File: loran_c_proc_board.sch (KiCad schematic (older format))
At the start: 28 parts, among them P101 Power, P102 Cortex SWD, P103 Clock board, U101 LD1117S33, U102 74AC14, U103 74AC14

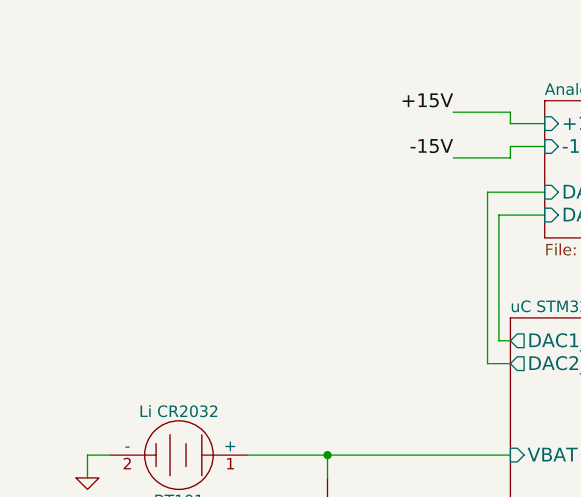
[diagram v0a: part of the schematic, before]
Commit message: Intermediate update #2: PCB routing/schematic tweaking in process
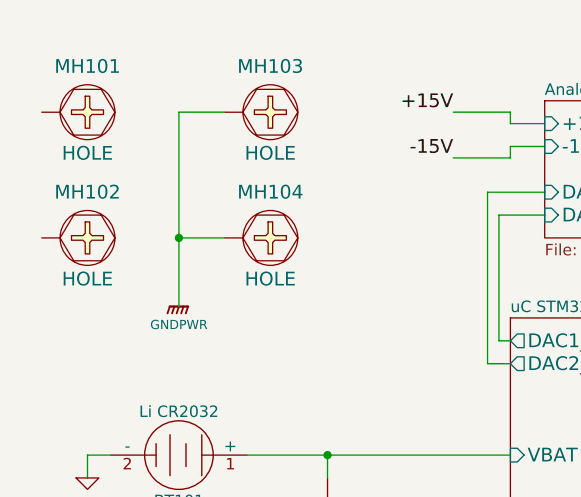
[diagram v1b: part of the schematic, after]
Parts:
- added MH101, MH102, MH103, MH104: HOLE, symbol HOLE
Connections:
- net GNDPWR: now also MH103.1, MH104.1
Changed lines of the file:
@@
 LIBS:transf
 LIBS:video
+LIBS:led_holder
 LIBS:loran_c_proc_board-cache
 EELAYER 24 0
@@
 	4900 1300 4900 1450
 Connection ~ 5300 1450
+$Comp
+L HOLE MH104
+U 1 1 52EF52BD
+P 1800 1800
+F 0 "MH104" H 1800 2000 60  0000 C CNN
+F 1 "HOLE" H 1800 1620 60  0000 C CNN
+F 2 "" H 1800 1800 60  0000 C CNN
+F 3 "" H 1800 1800 60  0000 C CNN
+	1    1800 1800
+	1    0    0    -1
+$EndComp
+$Comp
+L HOLE MH103
+U 1 1 52EF53B0
+P 1800 1250
+F 0 "MH103" H 1800 1450 60  0000 C CNN
+F 1 "HOLE" H 1800 1070 60  0000 C CNN
+F 2 "" H 1800 1250 60  0000 C CNN
+F 3 "" H 1800 1250 60  0000 C CNN
+	1    1800 1250
+	1    0    0    -1
+$EndComp
+$Comp
+L HOLE MH101
+U 1 1 52EF7090
+P 1000 1250
+F 0 "MH101" H 1000 1450 60  0000 C CNN
+F 1 "HOLE" H 1000 1070 60  0000 C CNN
+F 2 "" H 1000 1250 60  0000 C CNN
+F 3 "" H 1000 1250 60  0000 C CNN
+	1    1000 1250
+	1    0    0    -1
+$EndComp
+$Comp
+L HOLE MH102
+U 1 1 52EF741F
+P 1000 1800
+F 0 "MH102" H 1000 2000 60  0000 C CNN
+F 1 "HOLE" H 1000 1620 60  0000 C CNN
+F 2 "" H 1000 1800 60  0000 C CNN
+F 3 "" H 1000 1800 60  0000 C CNN
+	1    1000 1800
+	1    0    0    -1
+$EndComp
+$Comp
+L GNDPWR #PWR037
+U 1 1 52EF788F
+P 1400 2100
+F 0 "#PWR037" H 1400 2150 40  0001 C CNN
+F 1 "GNDPWR" H 1400 2020 40  0000 C CNN
+F 2 "" H 1400 2100 60  0000 C CNN
+F 3 "" H 1400 2100 60  0000 C CNN
+	1    1400 2100
+	1    0    0    -1
+$EndComp
+Wire Wire Line
+	1600 1800 1400 1800
+Wire Wire Line
+	1400 1250 1400 2100
+Wire Wire Line
+	1600 1250 1400 1250
+Connection ~ 1400 1800
 $EndSCHEMATC
